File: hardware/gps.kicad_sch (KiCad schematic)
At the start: 33 parts, among them Q4 BC817W, Q5 BC817W, U29 L96-M33

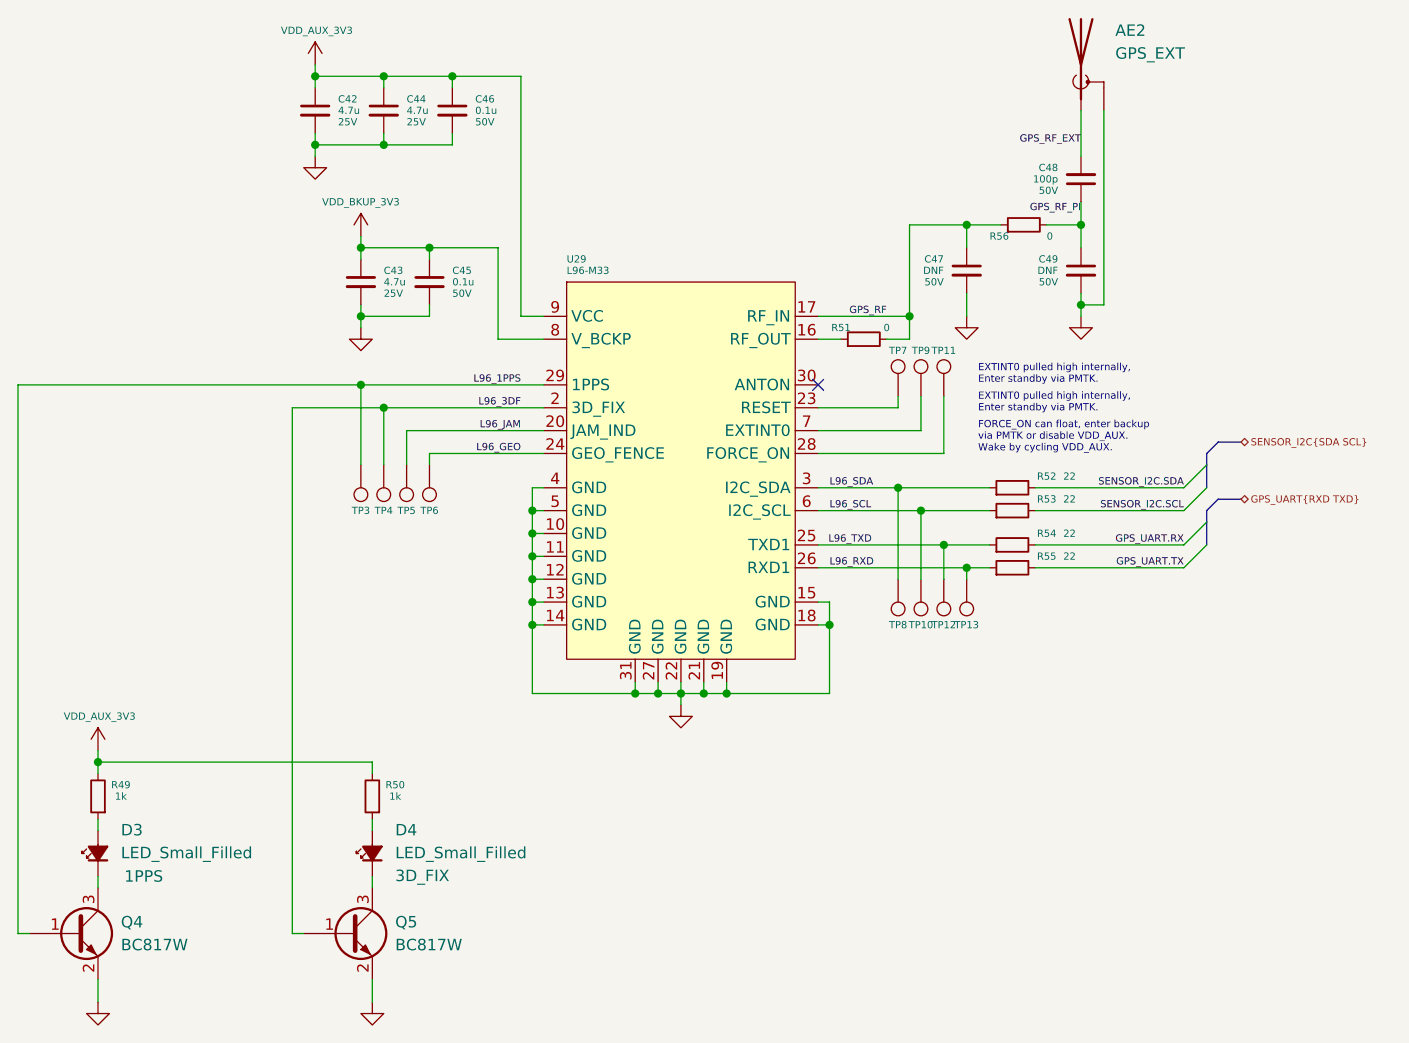
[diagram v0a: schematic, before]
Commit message: hardware update
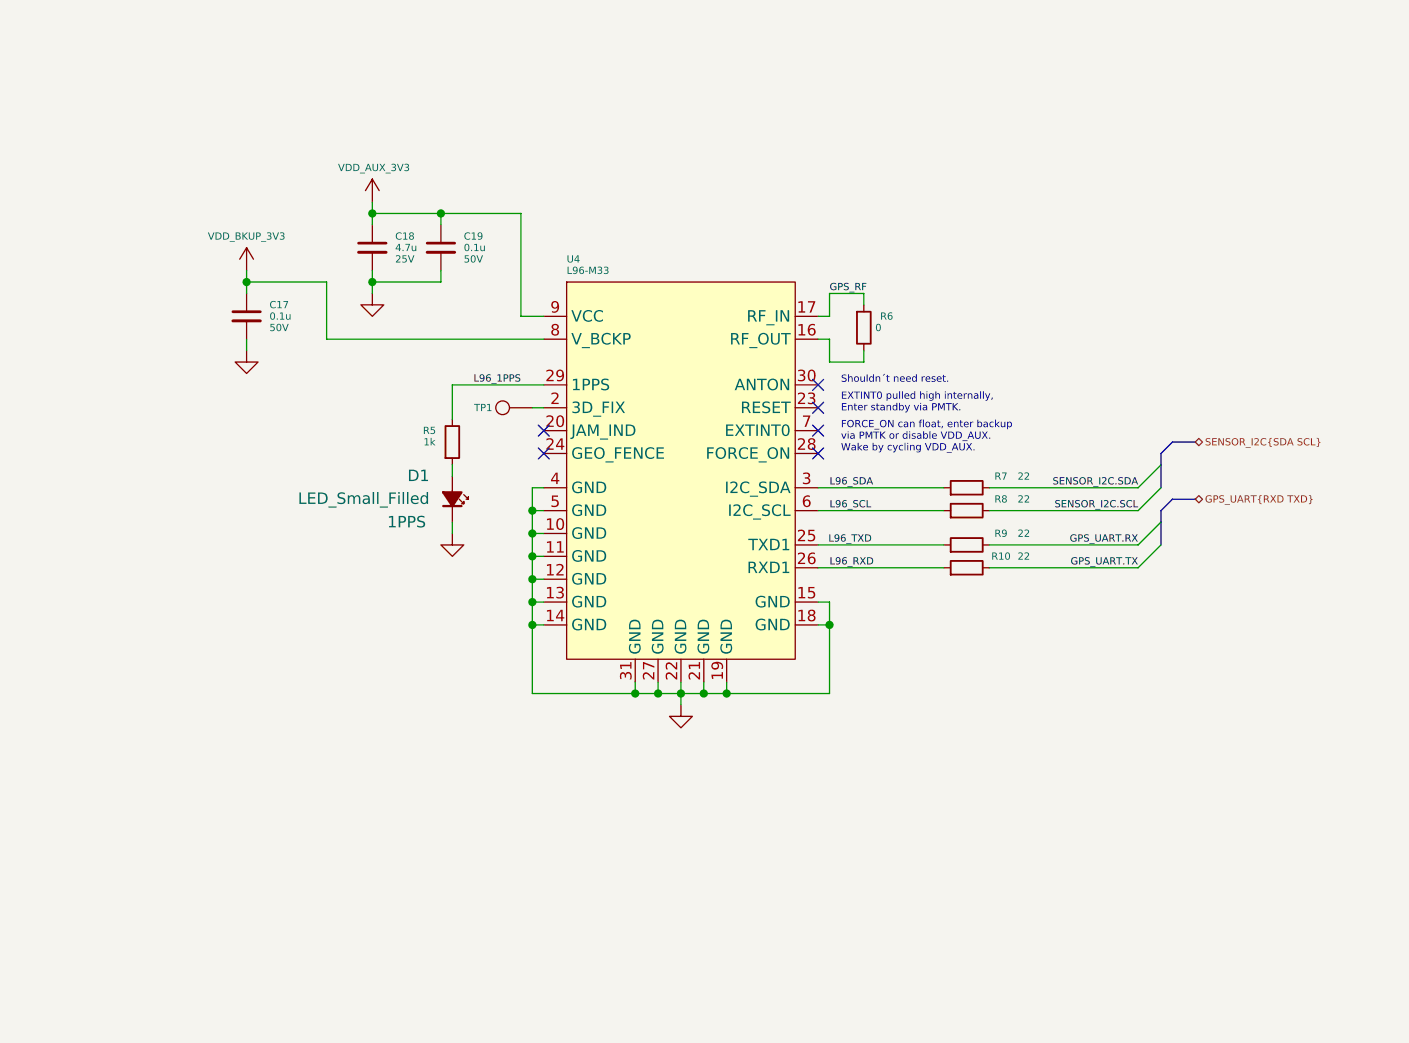
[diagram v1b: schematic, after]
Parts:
- removed AE2: GPS_EXT, Connector_Coaxial:U.FL_Hirose_U.FL-R-SMT-1_Vertical, symbol Device:Antenna_Shield
- removed C43, C44: 4.7u, Capacitor_SMD:C_0805_2012Metric, symbol Device:C_Small
- removed C47, C49: DNF, Capacitor_SMD:C_0402_1005Metric, symbol Device:C_Small
- removed C48: 100p, Capacitor_SMD:C_0402_1005Metric, symbol Device:C_Small
- removed D4: LED_Small_Filled, LED_SMD:LED_0603_1608Metric, symbol Device:LED_Small_Filled
- removed Q4, Q5: BC817W, Package_TO_SOT_SMD:SOT-323_SC-70, symbol Transistor_BJT:BC817W
- removed R50: 1k, Resistor_SMD:R_0603_1608Metric, symbol Device:R_Small
- removed R56: 0, Resistor_SMD:R_0402_1005Metric, symbol Device:R_Small
- removed TP10: L96_SCL, TestPoint:TestPoint_Pad_1.5x1.5mm, symbol Connector:TestPoint
- removed TP11: GPS_FORCE_ON, TestPoint:TestPoint_Pad_1.5x1.5mm, symbol Connector:TestPoint
- removed TP12: L96_TXD, TestPoint:TestPoint_Pad_1.5x1.5mm, symbol Connector:TestPoint
- removed TP13: L96_RXD, TestPoint:TestPoint_Pad_1.5x1.5mm, symbol Connector:TestPoint
- removed TP3, TP4, TP5: L96_JAM, TestPoint:TestPoint_Pad_1.5x1.5mm, symbol Connector:TestPoint
- removed TP6: L96_GEO, TestPoint:TestPoint_Pad_1.5x1.5mm, symbol Connector:TestPoint
- removed TP7: GPS_RESET, TestPoint:TestPoint_Pad_1.5x1.5mm, symbol Connector:TestPoint
- removed TP8: L96_SDA, TestPoint:TestPoint_Pad_1.5x1.5mm, symbol Connector:TestPoint
- removed TP9: GPS_EXTINT, TestPoint:TestPoint_Pad_1.5x1.5mm, symbol Connector:TestPoint
- added TP1: L96_FIX, TestPoint:TestPoint_Pad_D1.0mm, symbol Connector:TestPoint
- C17: renamed from C45; footprint Capacitor_SMD:C_0603_1608Metric -> Capacitor_SMD:C_0402_1005Metric
- C18: renamed from C42; footprint Capacitor_SMD:C_0805_2012Metric -> Capacitor_SMD:C_0603_1608Metric
- C19: renamed from C46; footprint Capacitor_SMD:C_0603_1608Metric -> Capacitor_SMD:C_0402_1005Metric
- R10: renamed from R55; footprint Resistor_SMD:R_0603_1608Metric -> Resistor_SMD:R_0402_1005Metric
- R5: renamed from R49; footprint Resistor_SMD:R_0603_1608Metric -> Resistor_SMD:R_0402_1005Metric
- R7: renamed from R52; footprint Resistor_SMD:R_0603_1608Metric -> Resistor_SMD:R_0402_1005Metric
- R8: renamed from R53; footprint Resistor_SMD:R_0603_1608Metric -> Resistor_SMD:R_0402_1005Metric
- R9: renamed from R54; footprint Resistor_SMD:R_0603_1608Metric -> Resistor_SMD:R_0402_1005Metric
- renumbered D3 to D1, R51 to R6, U29 to U4
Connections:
- net GND: now also D1.1 (K)
- net GPS_RF: now also R6.1; no longer R6.2
- net L96_1PPS: now also R5.2
- net VDD_AUX_3V3: no longer R5.2
- net at U4.16 (RF_OUT): now also R6.2; no longer R6.1
- net L96_3DF: no longer names the net of U4.2 (3D_FIX)
- net L96_3DF: now also TP1.1
- net L96_GEO: no longer names the net of U4.24 (GEO_FENCE)
- net L96_JAM: no longer names the net of U4.20 (JAM_IND)
- no-connect marks 1 -> 6
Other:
- note added: "Shouldn´t need reset."
- moved on the sheet: C17, C18, C19, D1, R10, R5, R6, R7, R8, R9
